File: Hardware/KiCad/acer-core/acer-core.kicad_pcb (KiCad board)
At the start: 4 copper layers, 31.5 x 36.9 mm, 18 parts, among them J1 Conn_01x14_Pin, J2 Conn_01x14_Pin, SW1 RESET, SW2 USER, U1 ESP32-S3-WROOM-1, U2 WIO-SX1262

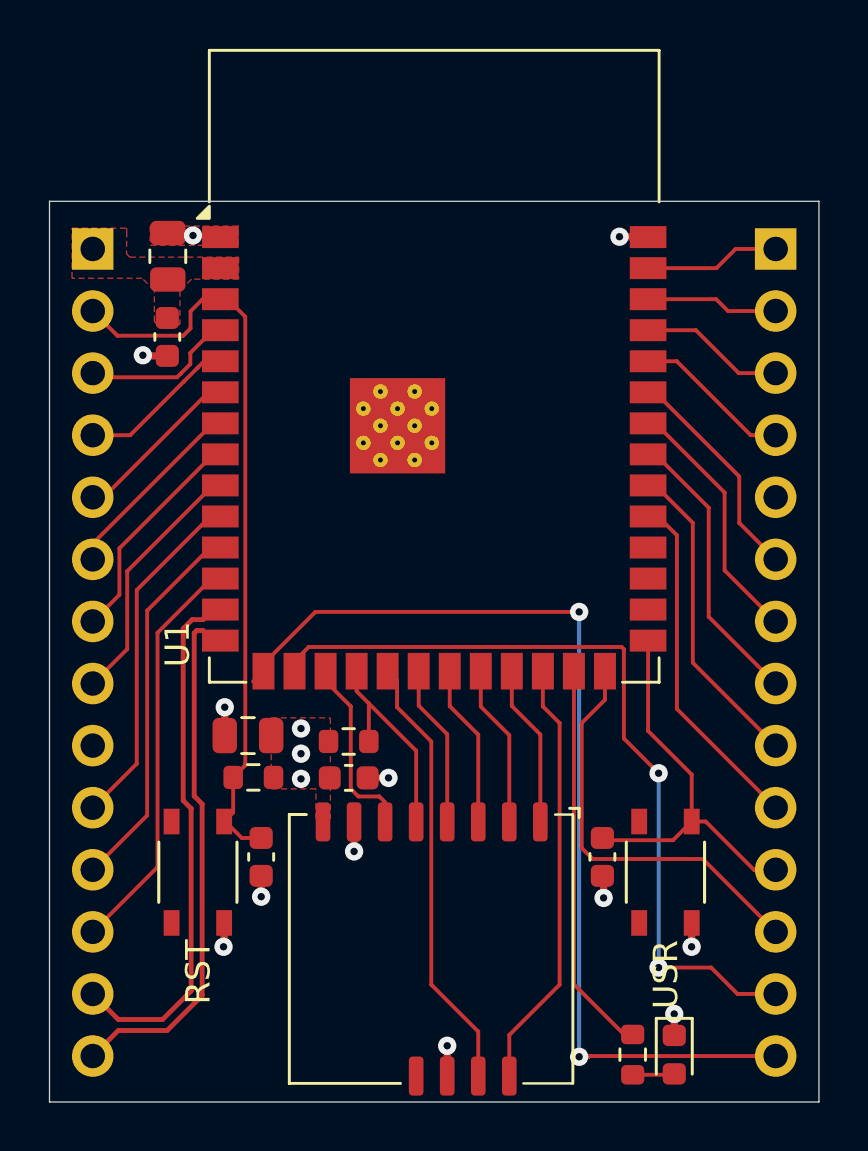
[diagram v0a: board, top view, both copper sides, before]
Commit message: Routing Done
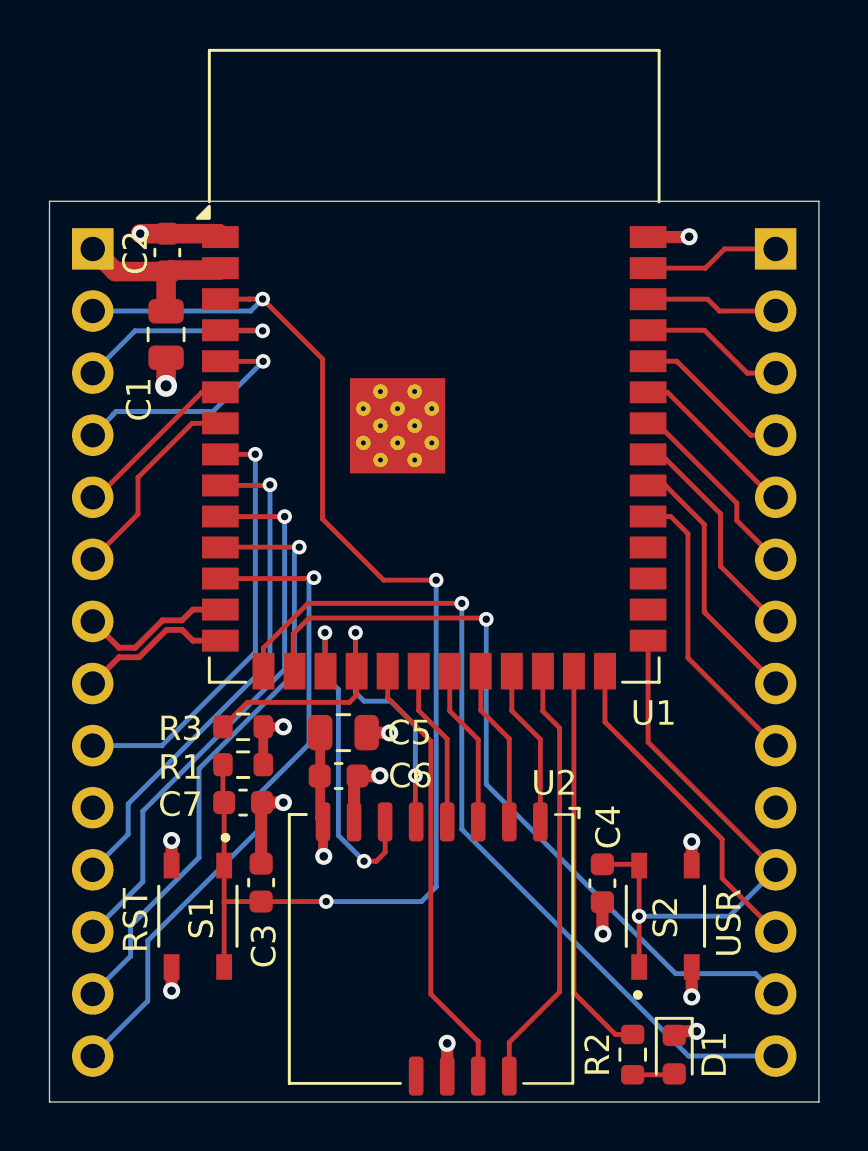
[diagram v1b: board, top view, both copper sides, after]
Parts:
- removed the G*** at (138.5, 94.8)
- removed SW1: RESET, SB_Button_Switch_SMD:SW_SKRPABE010
- removed SW2: USER, SB_Button_Switch_SMD:SW_SKRPABE010
- added C7: 1uF, Capacitor_SMD:C_0603_1608Metric, F.Cu at (130.7, 103.7)
- added G***: LOGO, SB-Logos:EG_Logo2_15mm_SilkScreen, B.Cu at (138.5, 88.4)
- added S1: RESET, SB_Button_Switch_SMD:SW_SKRPABE010, F.Cu at (128.8, 108.3)
- added S2: USER, SB_Button_Switch_SMD:SW_SKRPABE010, F.Cu at (147.9, 108.3)
- U1: value ESP32-S3-WROOM-1 -> ESP32-S3-WROOM-1-N4
- moved R3 4.36 mm to (130.7, 100.5), turned to 0 degrees
- moved C5 3.91 mm to (134.8, 100.8), turned to 0 degrees
- moved C2 3.45 mm to (127.5, 81.2), turned to 90 degrees
- moved C1 3.20 mm to (127.5, 84.5), turned to -90 degrees
- moved C4 1.08 mm to (145.3, 107.0)
- moved C3 1.05 mm to (131.4, 106.9), turned to 90 degrees
- moved R1 0.67 mm to (130.7, 102.1)
- moved C6 0.42 mm to (134.6, 102.6)
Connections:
- J1 pad 10: /IO17 -> GND
- J1 pad 11: /IO18 -> /IO16
- J1 pad 12: /IO8 -> /IO17
- J1 pad 13: /USB_D- -> /IO18
- J1 pad 14: /USB_D+ -> /IO8
- J1 pad 7: /IO15 -> /USB_D-
- J1 pad 8: /IO16 -> /USB_D+
- J1 pad 9: GND -> /IO15
- J2 pad 10: /IO38 -> GND
- J2 pad 5: GND -> /IO42
- J2 pad 6: /IO42 -> /IO41
- J2 pad 7: /IO41 -> /IO40
- J2 pad 8: /IO40 -> /IO39
- J2 pad 9: /IO39 -> /IO38
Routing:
- net /EN: track 31.3 -> 54.4 mm, vias 0 -> 3
- net /USB_D+: track 21.7 -> 6.31 mm
- net /USB_D-: track 21.7 -> 6.31 mm
- net +3.3V: track 0.00 -> 14.9 mm, vias 3 -> 2
- net /IO16: track 10.4 -> 20.8 mm, vias 0 -> 1
- net /IO8: track 17.2 -> 27.2 mm, vias 0 -> 1
- net GND: track 11.3 -> 21.2 mm, vias 12 -> 13
- net /IO18: track 15.6 -> 25.0 mm, vias 0 -> 1
- net /~{LORA_RST}: track 8.73 -> 18.0 mm, vias 0 -> 2
- net /IO15: track 9.17 -> 17.8 mm, vias 0 -> 1
- net /IO17: track 14.3 -> 22.9 mm, vias 0 -> 1
- net /USER: track 17.1 -> 23.6 mm, vias 0 -> 1
- net /LORA_NSS: track 7.68 -> 13.9 mm, vias 0 -> 2
- net /IO3: track 41.0 -> 35.7 mm, vias 2 -> 1
- net /IO5: track 6.47 -> 9.98 mm, vias 0 -> 1
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- added copper zone on In2.Cu, net +3.3V
- added copper zone on In1.Cu, net GND
- removed copper zone on F.Cu, net +3.3V
- removed copper zone on In1.Cu, net +3.3V
- removed copper zone on F.Cu, net GND
- removed copper zone on In2.Cu, net GND
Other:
- board text added: "AcerCore"
- board text added: "v1.1"
- board text removed: "v1.0"
